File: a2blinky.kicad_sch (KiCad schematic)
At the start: 28 parts, among them J1 Barrel_Jack_Switch, J2 Conn_01x02_Male, U1 74HC164, U2 4002, U3 AP1117-33, U4 LMC555xM

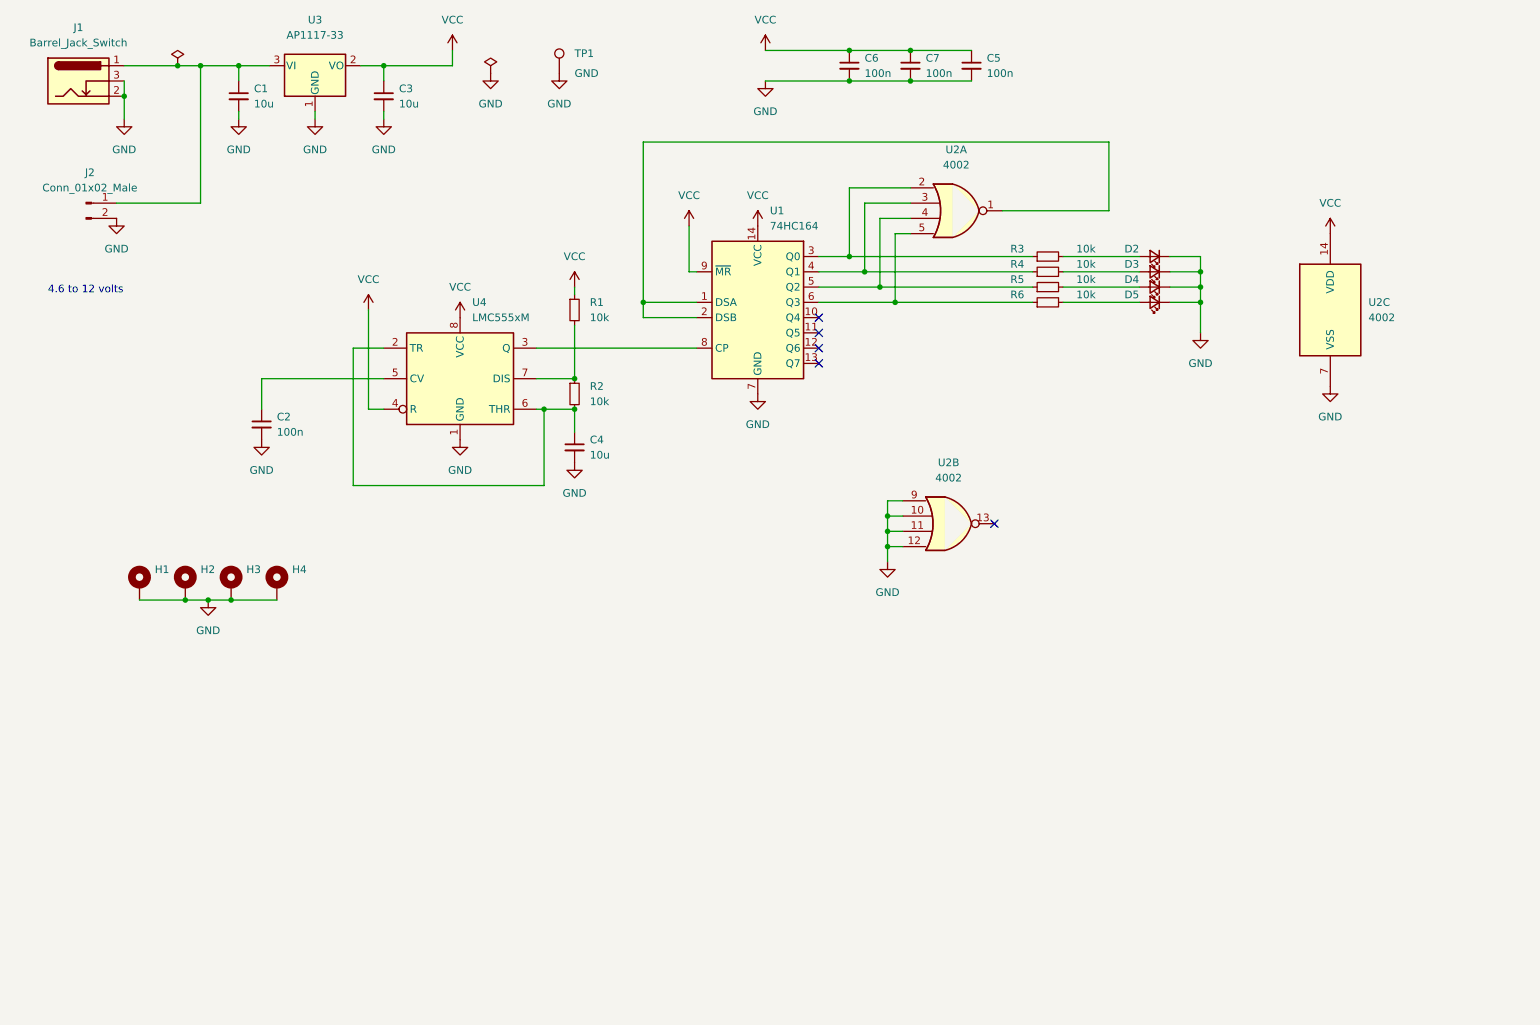
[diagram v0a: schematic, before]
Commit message: step3
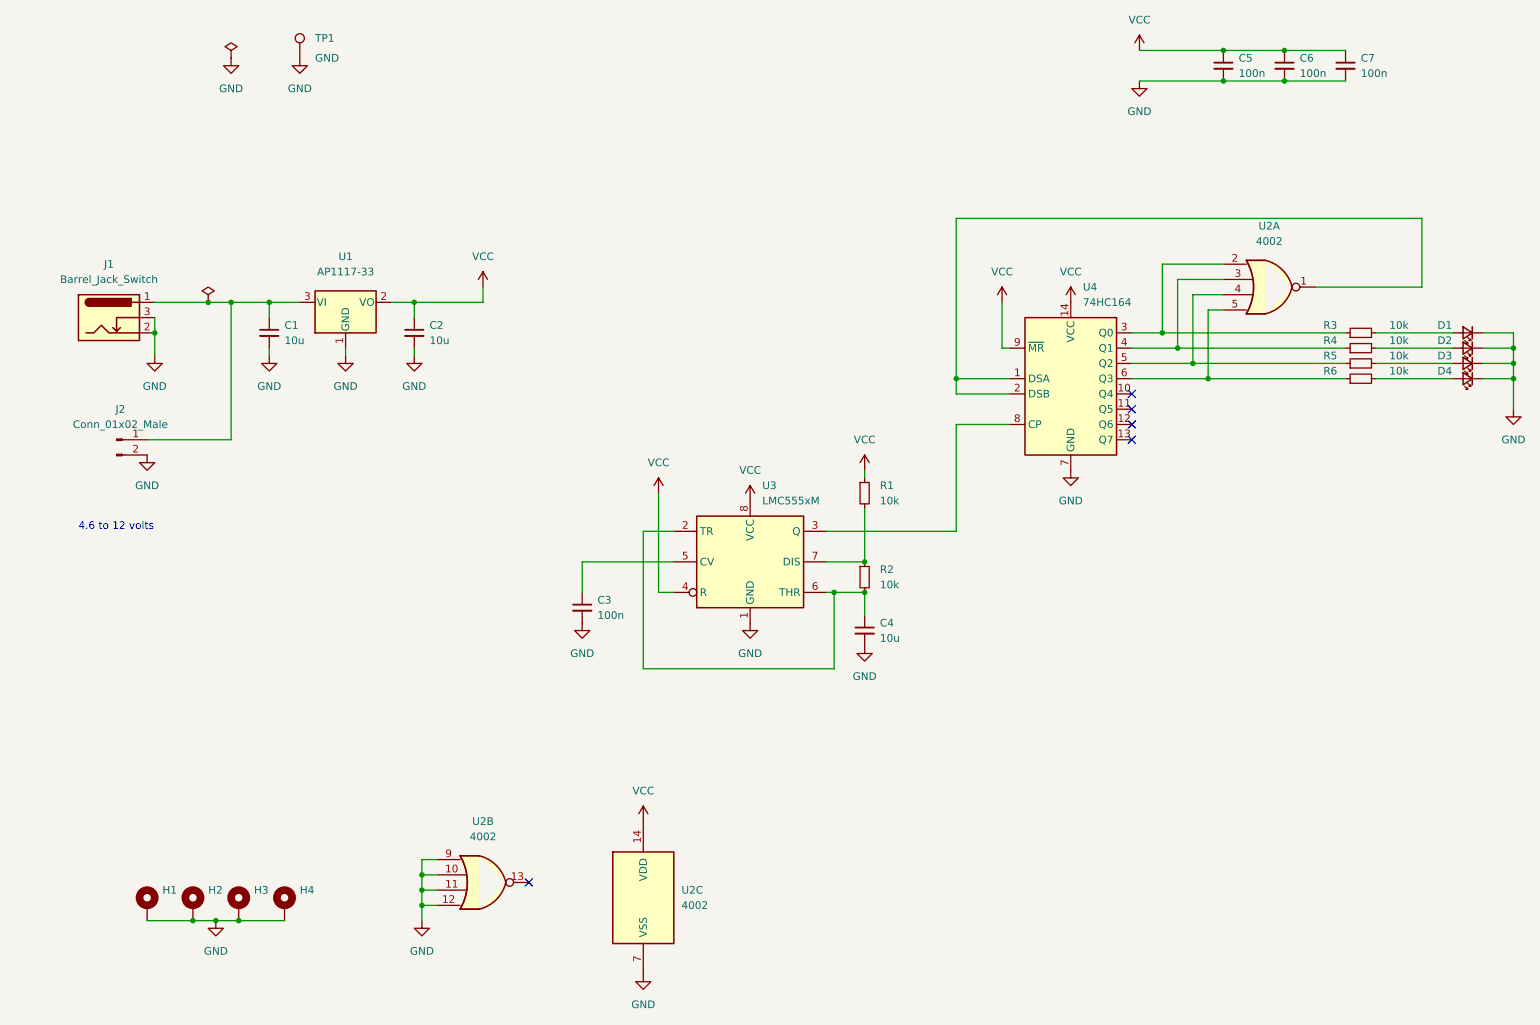
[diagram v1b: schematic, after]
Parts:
- renumbered C3 to C2, C2 to C3, C6 to C5, C7 to C6, C5 to C7, D2 to D1, D3 to D2, D4 to D3, D5 to D4, U3 to U1, U4 to U3, U1 to U4
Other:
- moved on the sheet: C1, C2, C3, C4, C5, C6, C7, D1, D2, D3, D4, H1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
